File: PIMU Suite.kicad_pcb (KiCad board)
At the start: 2 copper layers, 77 x 50.5 mm, 16 parts, among them U2 MICROSD_SPI_OR_SDIO_CARD

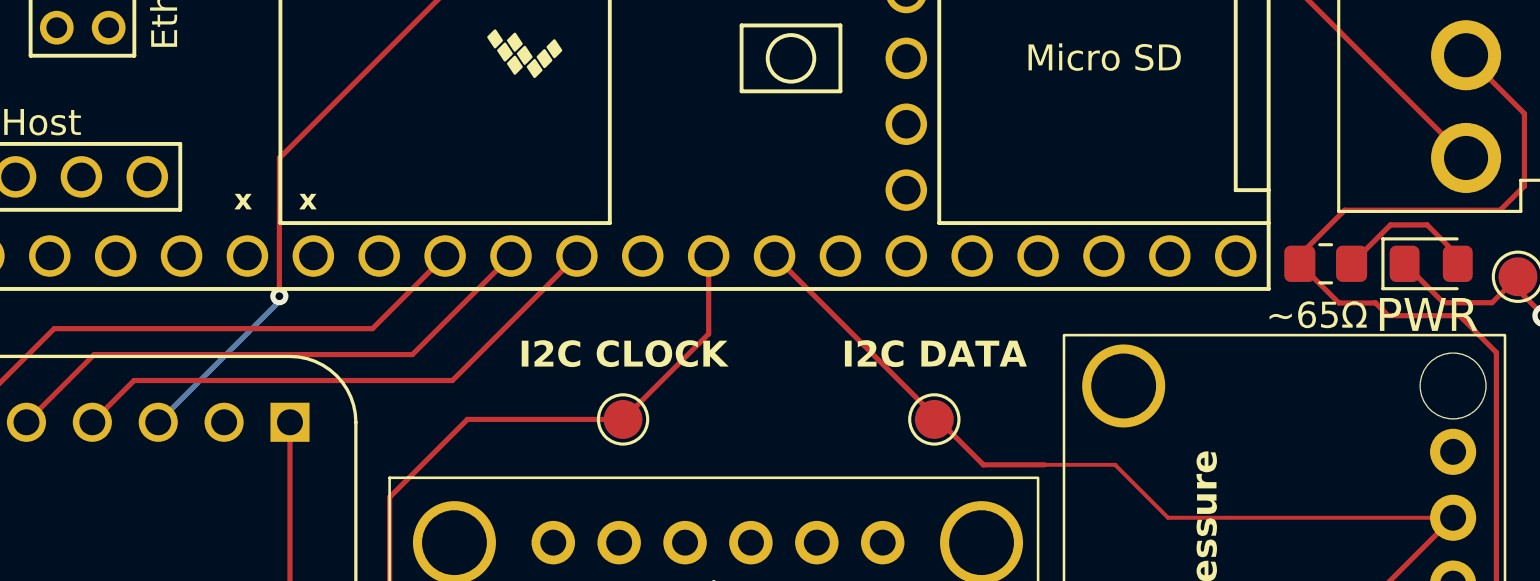
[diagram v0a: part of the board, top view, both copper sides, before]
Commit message: JLCPCB specs
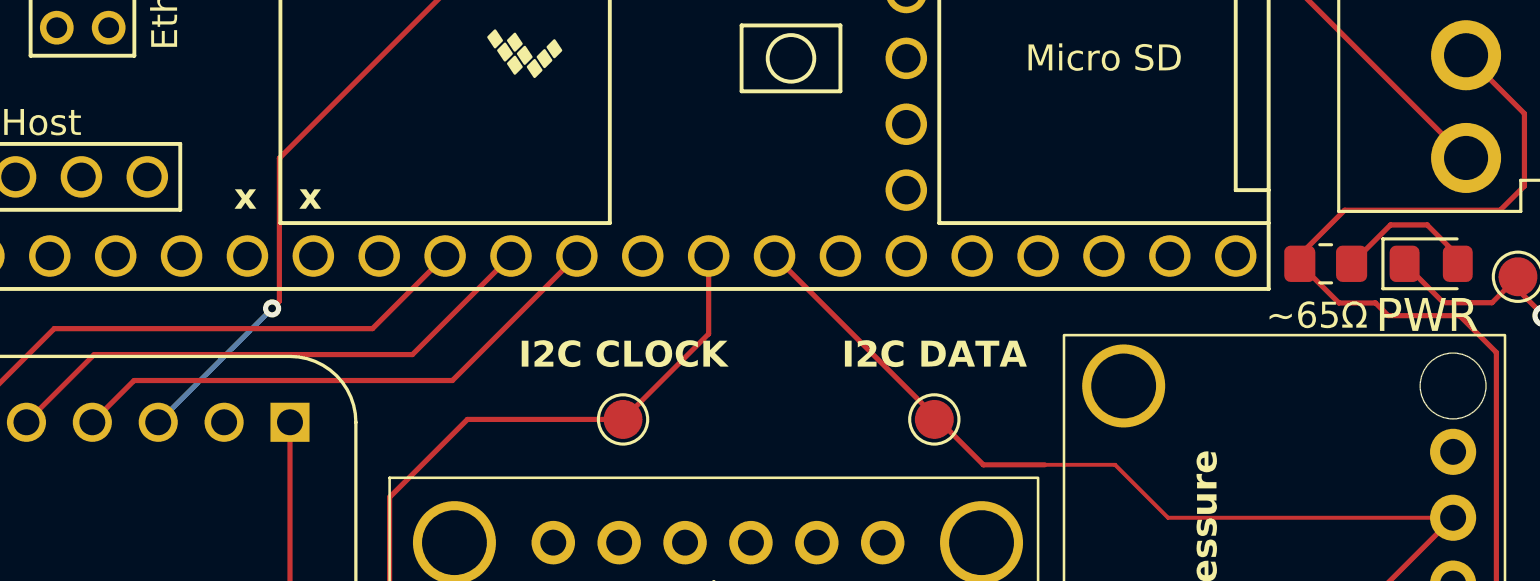
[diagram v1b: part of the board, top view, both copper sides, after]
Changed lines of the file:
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@@
 		)
 		(pad_to_mask_clearance 0)
+		(solder_mask_min_width 0.12)
 		(allow_soldermask_bridges_in_footprints no)
 		(tenting front back)
 		(pcbplotparams
 			(layerselection 0x00000000_00000000_55555555_5755f5ff)
-			(plot_on_all_layers_selection 0x00000000_00000000_00000000_0200a0af)
+			(plot_on_all_layers_selection 0x00000000_00000000_00000000_00000000)
 			(disableapertmacros no)
 			(usegerberextensions no)
@@
 			(dashed_line_gap_ratio 3.000000)
 			(svgprecision 4)
-			(plotframeref yes)
+			(plotframeref no)
 			(mode 1)
 			(useauxorigin no)
@@
 			(pdf_back_fp_property_popups yes)
 			(pdf_metadata yes)
-			(pdf_single_document yes)
+			(pdf_single_document no)
 			(dxfpolygonmode yes)
 			(dxfimperialunits yes)
@@
 			(psnegative no)
 			(psa4output no)
-			(plot_black_and_white no)
+			(plot_black_and_white yes)
 			(sketchpadsonfab no)
 			(plotpadnumbers no)
@@
 			(crossoutdnponfab yes)
 			(subtractmaskfromsilk no)
-			(outputformat 4)
+			(outputformat 1)
 			(mirror no)
 			(drillshape 0)
 			(scaleselection 1)
-			(outputdirectory "Board Versions/")
+			(outputdirectory "Drills/")
 		)
 	)
@@
 				(font
 					(size 1 1)
-					(thickness 0.125)
+					(thickness 0.15)
 				)
 			)
@@
 		(effects
 			(font
-				(size 0.8 0.8)
+				(size 1 1)
 				(thickness 0.1875)
 				(bold yes)
@@
 		(effects
 			(font
-				(size 0.8 0.8)
+				(size 1 1)
 				(thickness 0.1875)
 				(bold yes)
@@
 	)
 	(segment
+		(start 131.75 95.44)
+		(end 131.75 89.93)
+		(width 0.2)
+		(layer "F.Cu")
+		(net 19)
+	)
+	(segment
 		(start 127.08 100.11)
 		(end 127.08 99.92)
@@
 	)
 	(segment
-		(start 131.75 89.93)
-		(end 143.22 78.46)
+		(start 131.47 95.72)
+		(end 131.75 95.44)
 		(width 0.2)
 		(layer "F.Cu")
@@
 	)
 	(segment
-		(start 131.75 95.25)
-		(end 131.75 89.93)
+		(start 131.75 89.93)
+		(end 143.22 78.46)
 		(width 0.2)
 		(layer "F.Cu")
@@
 	)
 	(via
-		(at 131.75 95.25)
+		(at 131.47 95.72)
 		(size 0.7)
 		(drill 0.3)
@@
 	)
 	(segment
-		(start 131.75 95.25)
-		(end 131.75 95.44)
+		(start 131.47 95.72)
+		(end 127.08 100.11)
 		(width 0.2)
 		(layer "B.Cu")
@@
 		(width 0.2)
 		(layer "B.Cu")
-		(net 19)
-	)
-	(segment
-		(start 131.75 95.44)
-		(end 127.08 100.11)
-		(width 0.2)
-		(layer "B.Cu")
